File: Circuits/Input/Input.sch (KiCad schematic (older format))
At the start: 9 parts, among them J1 sensor, P1 WRITER-VCC, SW1 MKA-10110, U1 TWELITE_SMD

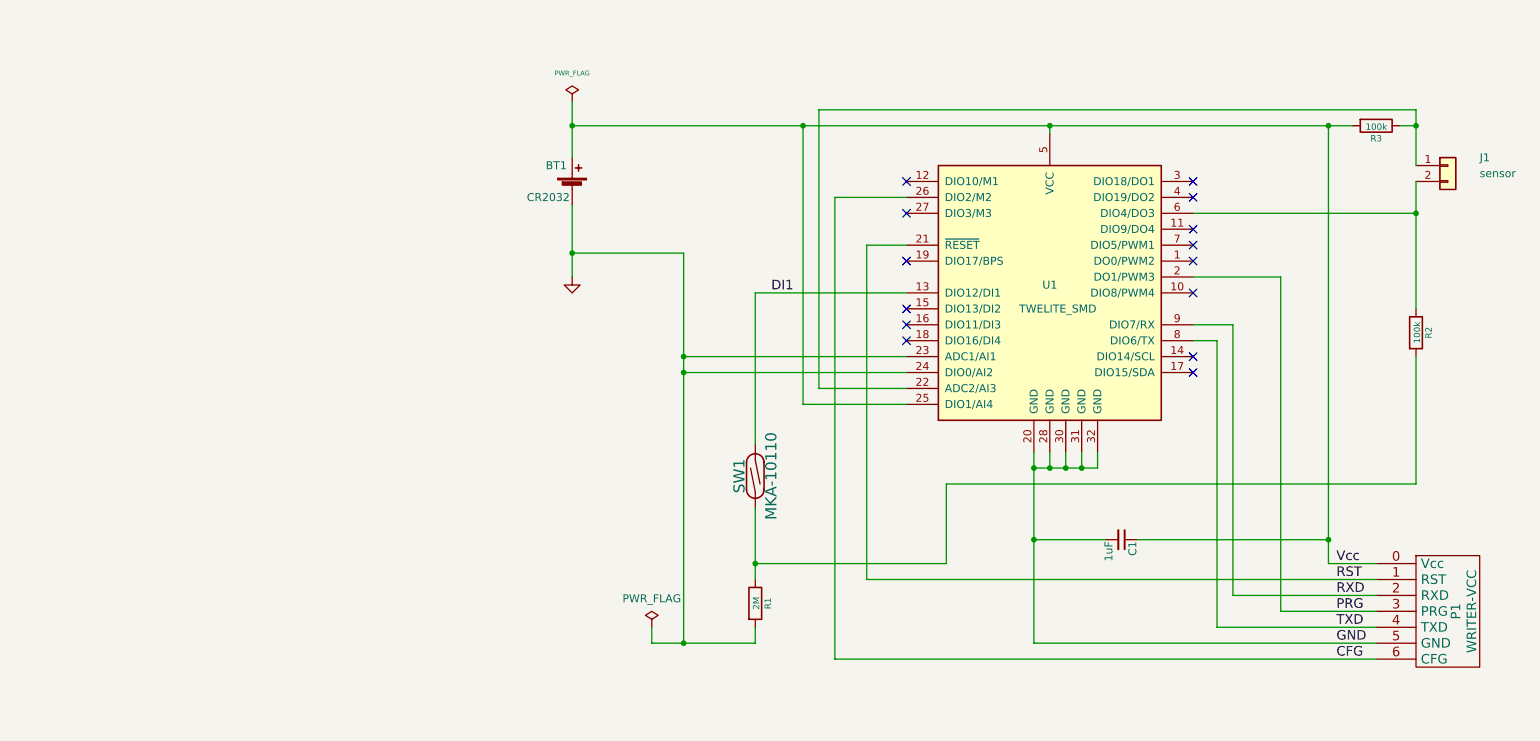
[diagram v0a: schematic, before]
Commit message: Updated footprint
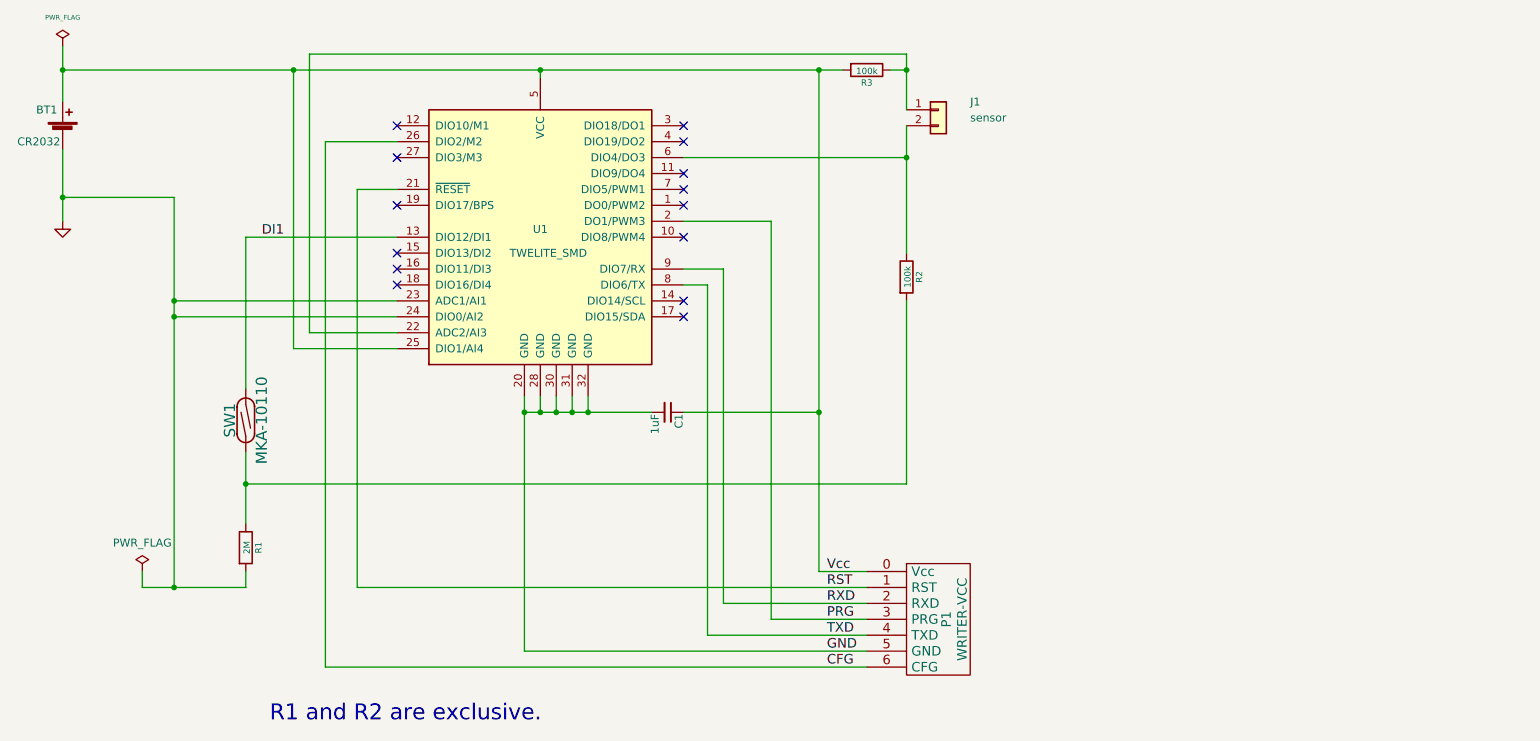
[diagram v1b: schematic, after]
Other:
- note added: "R1 and R2 are exclusive."
- moved on the sheet: BT1, C1, J1, P1, R1, R2, R3, SW1, U1

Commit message: Updated symbols
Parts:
- U1: symbol RF_ZigBee:TWELITE_SMD -> RF_ZigBee:TWELITE
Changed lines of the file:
@@
-	1    0    0    -1
-$EndComp
-$Comp
-L power:PWR_FLAG #FLG02
-U 1 1 5486A030
-P 1250 1250
-F 0 "#FLG02" H 1250 1345 30  0001 C CNN
-F 1 "PWR_FLAG" H 1250 1430 30  0000 C CNN
-F 2 "" H 1250 1250 60  0000 C CNN
-F 3 "" H 1250 1250 60  0000 C CNN
-	1    1250 1250
 	1    0    0    -1
 $EndComp
@@
 	1    0    0    -1
 $EndComp
-NoConn ~ 3350 1750
+NoConn ~ 3450 1750
 Text Label 2500 2450 0    60   ~ 0
 DI1
-NoConn ~ 3350 1950
+NoConn ~ 3450 1950
 Text Label 6050 4650 0    60   ~ 0
 RST
 Text Label 6050 4850 0    60   ~ 0
 PRG
-$Comp
-L power:PWR_FLAG #FLG03
-U 1 1 550F8F4A
-P 1750 4550
-F 0 "#FLG03" H 1750 4645 50  0001 C CNN
-F 1 "PWR_FLAG" H 1750 4730 50  0000 C CNN
-F 2 "" H 1750 4550 60  0000 C CNN
-F 3 "" H 1750 4550 60  0000 C CNN
-	1    1750 4550
-	1    0    0    -1
-$EndComp
 $Comp
 L Device:R R3
@@
 	6550 1750 6550 1950
 Wire Wire Line
-	5150 1950 6550 1950
+	5050 1950 6550 1950
 Connection ~ 1950 2950
 Wire Wire Line
-	1950 2950 3350 2950
-Connection ~ 1250 1400
+	1950 2950 3450 2950
 Wire Wire Line
 	1250 2200 1950 2200
@@
 	1250 1900 1250 2200
 Wire Wire Line
-	1250 1250 1250 1400
-Wire Wire Line
 	2700 1400 2700 3150
 Wire Wire Line
-	1750 4650 1950 4650
-Wire Wire Line
 	6000 4550 6300 4550
 Wire Wire Line
 	1250 1400 2700 1400
 Wire Wire Line
-	3350 2150 3100 2150
+	3450 2150 3100 2150
 Wire Wire Line
 	3100 2150 3100 4650
 Wire Wire Line
-	5150 2350 5700 2350
+	5050 2350 5700 2350
 Wire Wire Line
 	2900 1850 2900 5150
@@
 	2400 3400 2400 2450
 Wire Wire Line
-	2400 2450 3350 2450
-Wire Wire Line
-	2700 3150 3350 3150
-Wire Wire Line
-	3350 1850 2900 1850
+	2400 2450 3450 2450
+Wire Wire Line
+	2700 3150 3450 3150
+Wire Wire Line
+	3450 1850 2900 1850
 Wire Wire Line
 	2400 4650 2400 4550
@@
 	5700 4850 6300 4850
 Wire Wire Line
-	1750 4550 1750 4650
-Wire Wire Line
 	1950 2200 1950 2850
-Connection ~ 1950 4650
-Wire Wire Line
-	3350 2850 1950 2850
+Wire Wire Line
+	3450 2850 1950 2850
 Connection ~ 1950 2850
 Wire Wire Line
@@
 Wire Wire Line
 	2700 1400 4250 1400
-NoConn ~ 5150 1750
-NoConn ~ 5150 1850
-NoConn ~ 5150 2050
-NoConn ~ 5150 2850
-NoConn ~ 5150 2950
+NoConn ~ 5050 1750
+NoConn ~ 5050 1850
+NoConn ~ 5050 2050
+NoConn ~ 5050 2850
+NoConn ~ 5050 2950
 Wire Wire Line
 	4150 5050 6300 5050
@@
 $EndComp
 Wire Wire Line
-	5150 2750 5300 2750
+	5050 2750 5300 2750
 Wire Wire Line
 	5300 2750 5300 4950
@@
 	5300 4950 6300 4950
 Wire Wire Line
-	5150 2650 5400 2650
+	5050 2650 5400 2650
 Wire Wire Line
 	5400 2650 5400 4750
 Wire Wire Line
 	5400 4750 6300 4750
-NoConn ~ 5150 2150
-NoConn ~ 5150 2250
-NoConn ~ 5150 2450
-NoConn ~ 3350 2250
-Wire Wire Line
-	3350 3050 2800 3050
-NoConn ~ 3350 2550
-NoConn ~ 3350 2650
-NoConn ~ 3350 2750
+NoConn ~ 5050 2150
+NoConn ~ 5050 2250
+NoConn ~ 5050 2450
+NoConn ~ 3450 2250
+Wire Wire Line
+	3450 3050 2800 3050
+NoConn ~ 3450 2550
+NoConn ~ 3450 2650
+NoConn ~ 3450 2750
 Wire Wire Line
 	4250 1450 4250 1400
@@
 	5150 3550 6000 3550
 $Comp
-L RF_ZigBee:TWELITE_SMD U1
+L RF_ZigBee:TWELITE U1
 U 1 1 5A9FFEF1
 P 4250 2450
-F 0 "U1" H 4250 2500 50  0000 C CNN
-F 1 "TWELITE_SMD" H 4300 2350 50  0000 C CNN
+F 0 "U1" H 3800 3300 50  0000 C CNN
+F 1 "TWELITE_SMD" H 4550 3300 50  0000 C CNN
 F 2 "RF_Module:TWELITE_SMD" H 4250 1350 50  0001 C CNN
 F 3 "https://www.mono-wireless.com/jp/products/TWE-LITE/MW-PDS-TWELITE-JP.pdf" H 5000 1450 50  0001 C CNN
@@
 	2400 4000 6550 4000
 Connection ~ 4550 3550
+Connection ~ 1250 1400
+Wire Wire Line
+	1250 1250 1250 1400
+$Comp
+L power:PWR_FLAG #FLG02
+U 1 1 5486A030
+P 1250 1250
+F 0 "#FLG02" H 1250 1345 30  0001 C CNN
+F 1 "PWR_FLAG" H 1250 1430 30  0000 C CNN
+F 2 "" H 1250 1250 60  0000 C CNN
+F 3 "" H 1250 1250 60  0000 C CNN
+	1    1250 1250
+	1    0    0    -1
+$EndComp
+$Comp
+L power:PWR_FLAG #FLG?
+U 1 1 5AAF2C2D
+P 1750 4550
+F 0 "#FLG?" H 1750 4645 30  0001 C CNN
+F 1 "PWR_FLAG" H 1750 4730 30  0000 C CNN
+F 2 "" H 1750 4550 60  0000 C CNN
+F 3 "" H 1750 4550 60  0000 C CNN
+	1    1750 4550
+	1    0    0    -1
+$EndComp
+Wire Wire Line
+	1750 4550 1750 4650
+Wire Wire Line
+	1750 4650 1950 4650
+Connection ~ 1950 4650
 $EndSCHEMATC
